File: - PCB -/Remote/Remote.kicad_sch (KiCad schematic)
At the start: 49 parts, among them J1 Conn_01x02_Pin, J2 Conn_01x02_Pin, J3 Conn_01x02_Pin, J4 AVR-ISP-6, J5 Conn_01x02_Pin, Q1 NMOS, SW1 SW_Push, SW2 SW_Push, SW3 SW_Push, SW4 SW_DIP_x05, U1 ATmega168PA-A, Y1 Crystal

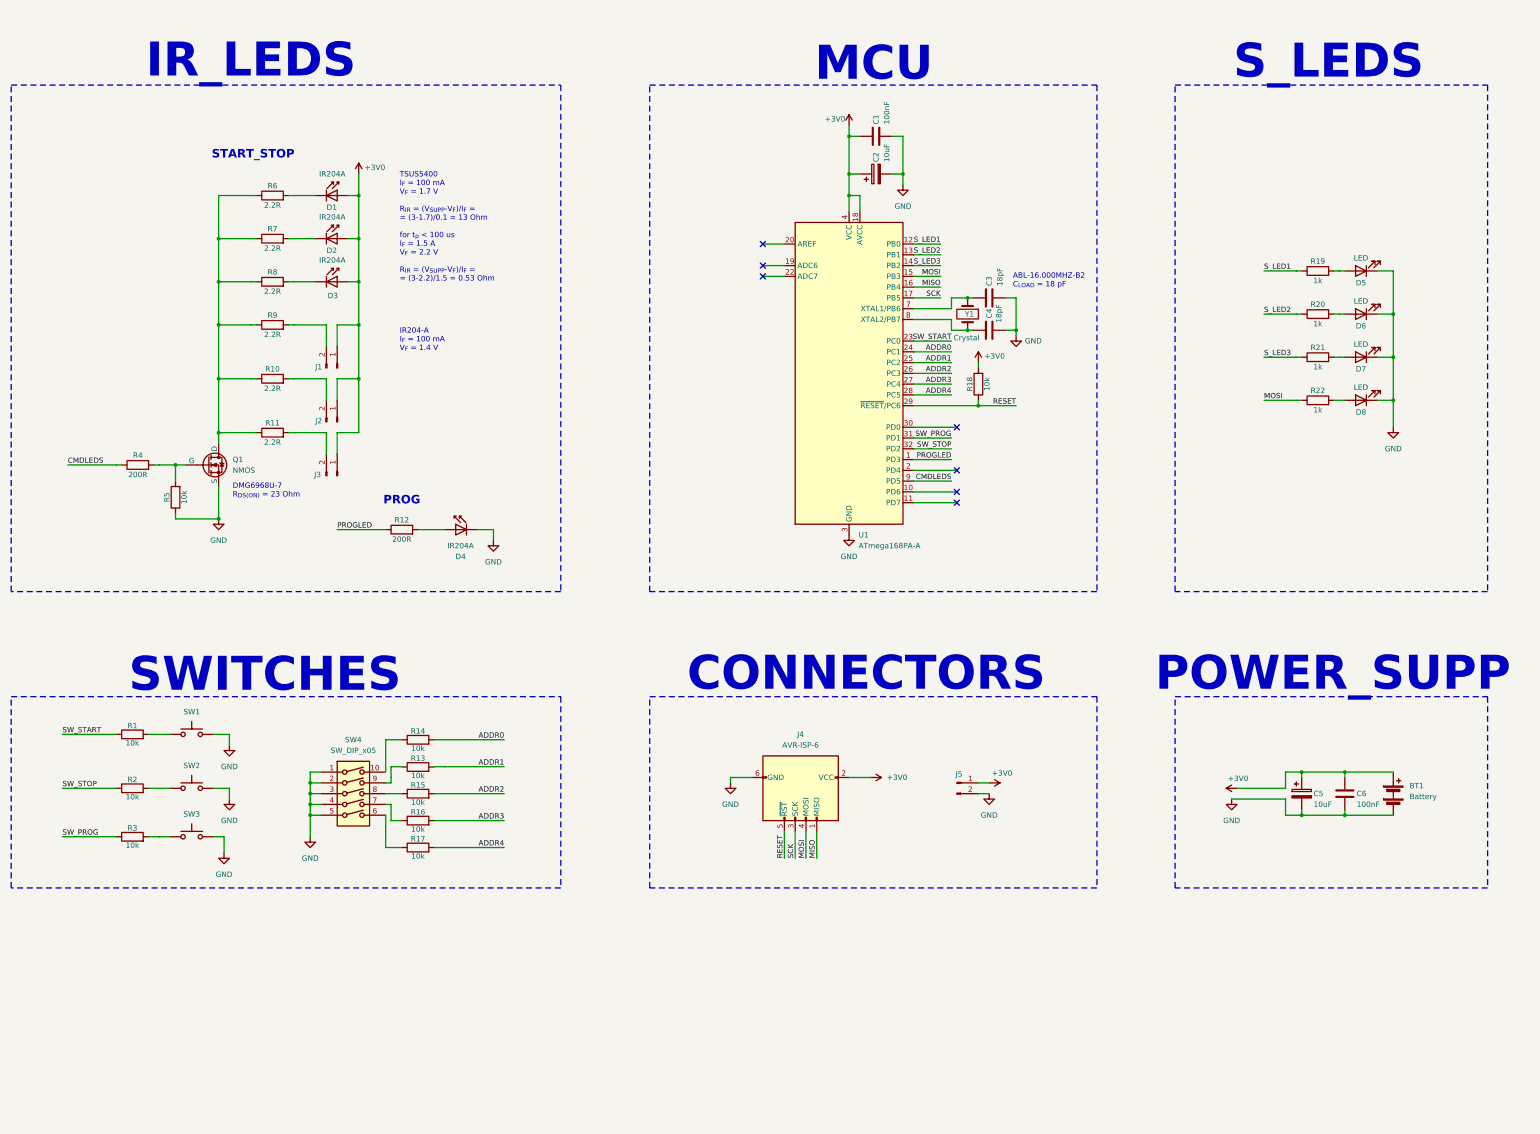
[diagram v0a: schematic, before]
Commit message: remote pcb
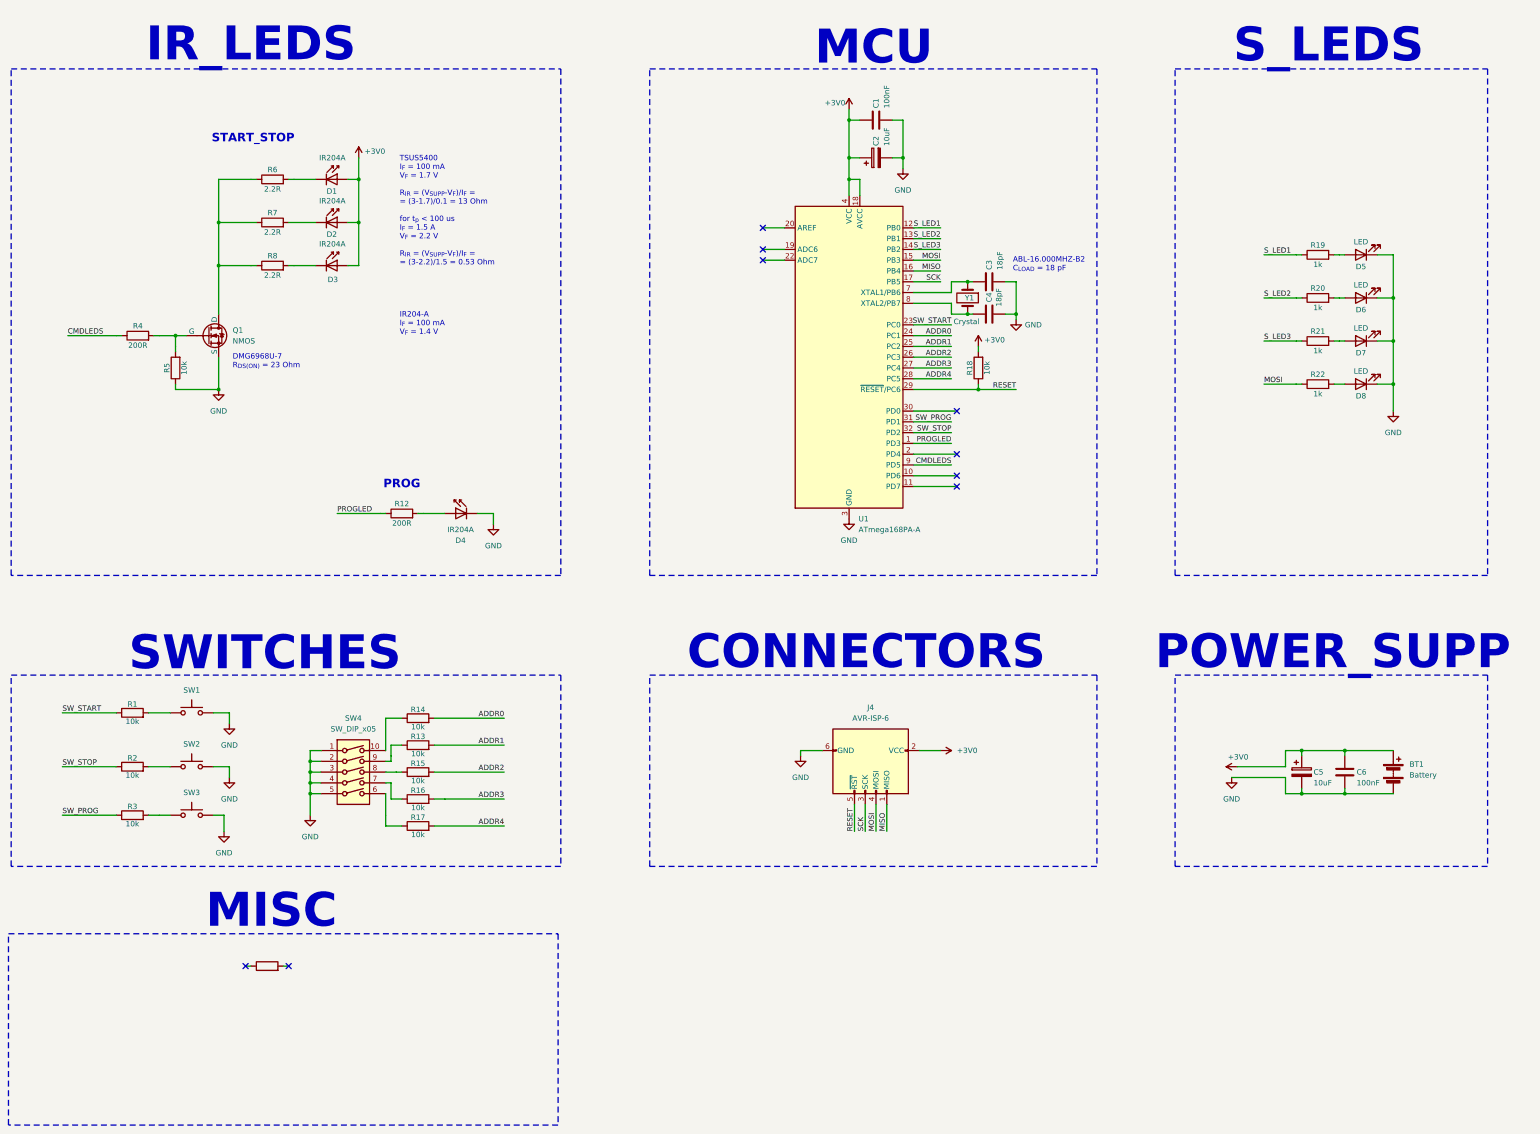
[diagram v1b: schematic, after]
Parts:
- removed J1, J2, J3, J5: Conn_01x02_Pin, Connector_PinHeader_2.54mm:PinHeader_1x02_P2.54mm_Vertical, symbol Connector:Conn_01x02_Pin
- removed R10, R11: 2.2R, Resistor_SMD:R_0805_2012Metric_Pad1.20x1.40mm_HandSolder, symbol Device:R
- R9: value 2.2R -> R; footprint Resistor_SMD:R_0805_2012Metric_Pad1.20x1.40mm_HandSolder -> sumec-remote_library:purosidenegative
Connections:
- net ADDR1: now also R13.2
- net at Q1.1 (D), R6.1, R7.1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: no longer R9.1
- net at SW4.9: now also R13.1
- no-connect marks 7 -> 9
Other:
- note added: "MISC"
- moved on the sheet: BT1, C1, C2, C3, C4, C5, C6, D1, D2, D3, D4, D5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
